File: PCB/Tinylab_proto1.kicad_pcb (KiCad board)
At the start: 2 copper layers, 36.8 x 34.7 mm, 79 parts, among them IC1 ATXMEGA32A4U-AU, P1 SCOPE_OUT, P10 EXPANSION, P11 SWITCH, P2 USB_OTG, P3 DIG_OUT, P4 PDI/3V3, P5 SCOPE_OUT, P6 DAC_OUT, P7 PSU, P8 DIG_IN, P9 FUSE_BYPASS, Q1 Q_NMOS_GSD, U1 78L05, U2 LM324, U3 DMN63D8LDW, U4 DMN63D8LDW

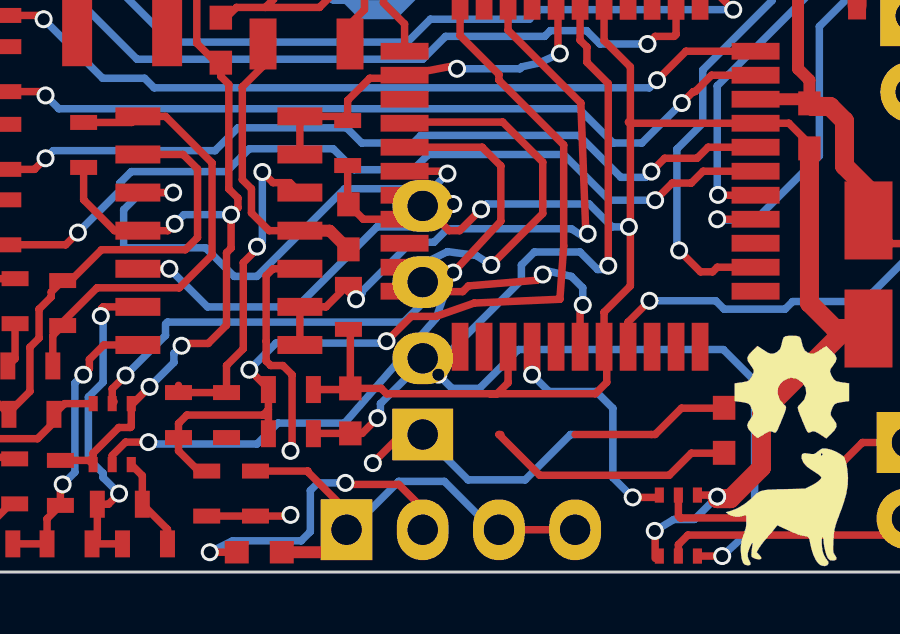
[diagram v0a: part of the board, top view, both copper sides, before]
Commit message: reverted PCB to genuine version
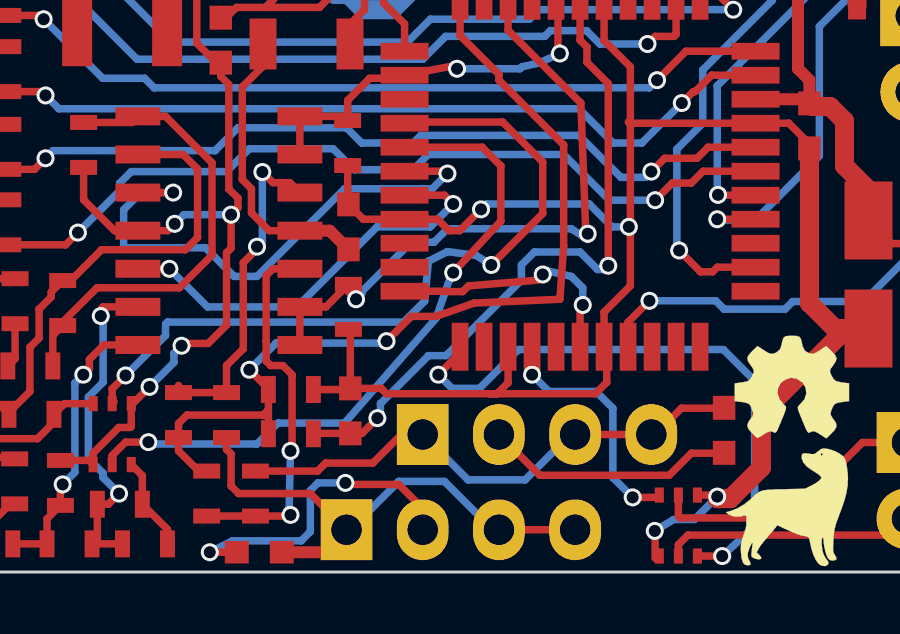
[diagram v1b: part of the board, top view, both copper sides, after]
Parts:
- turned P1 to 90 degrees
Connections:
- R1 pad 1: /Scope_Buffer_Input_CH2 -> /Scope_Buffer_Input_CH1
- R1 pad 2: /Scope_CH2_DC -> /Scope_CH1_DC
- R2 pad 2: /Scope_CH1_DC -> /Scope_CH2_DC
- R3 pad 1: /Scope_Buffer_Input_CH2 -> /Scope_Buffer_Input_CH1
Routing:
- net /Scope_Buffer_Input_CH1: track 7.68 -> 12.6 mm, vias 1 -> 2
- net /Scope_CH1_DC: track 13.4 -> 17.4 mm, vias 1 -> 0
- net /Scope_Buffer_Input_CH2: track 14.1 -> 11.2 mm, vias 3 -> 2
- net /Scope_CH2_DC: track 16.8 -> 18.9 mm
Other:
- net class Default added: clearance 0.2, trace_width 0.25, via_dia 0.6, via_drill 0.4

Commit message: removed commented code lines
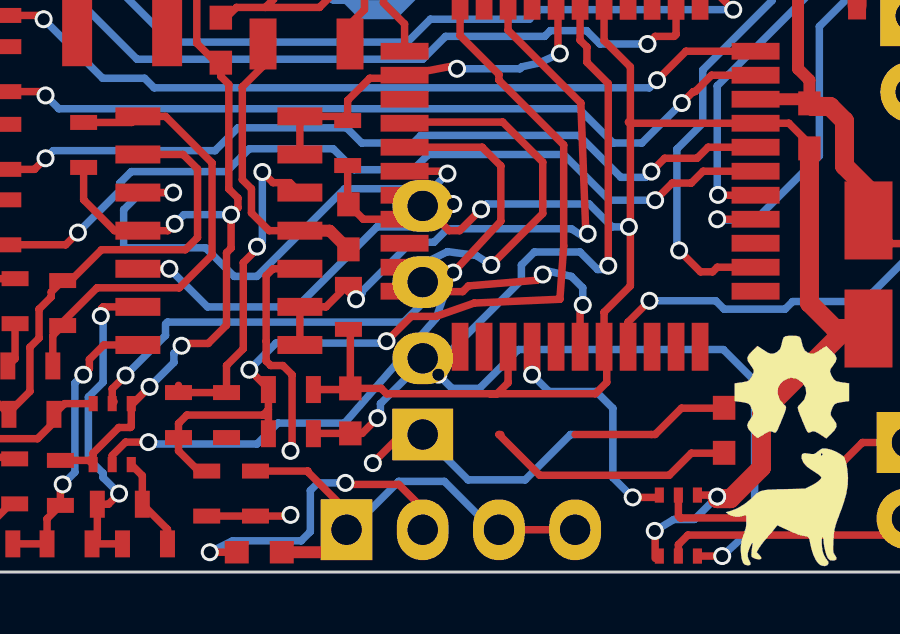
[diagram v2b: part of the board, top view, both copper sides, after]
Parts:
- turned P1 to 180 degrees
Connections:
- R1 pad 1: /Scope_Buffer_Input_CH1 -> /Scope_Buffer_Input_CH2
- R1 pad 2: /Scope_CH1_DC -> /Scope_CH2_DC
- R2 pad 2: /Scope_CH2_DC -> /Scope_CH1_DC
- R3 pad 1: /Scope_Buffer_Input_CH1 -> /Scope_Buffer_Input_CH2
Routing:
- net /Scope_Buffer_Input_CH1: track 12.6 -> 7.68 mm, vias 2 -> 1
- net /Scope_CH1_DC: track 17.4 -> 13.4 mm, vias 0 -> 1
- net /Scope_Buffer_Input_CH2: track 11.2 -> 14.1 mm, vias 2 -> 3
- net /Scope_CH2_DC: track 18.9 -> 16.8 mm
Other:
- net class Default removed
